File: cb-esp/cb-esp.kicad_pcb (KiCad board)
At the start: 4 copper layers, 25.4 x 55.8 mm, 24 parts, among them P1 CONN_01X07, P2 CONN_01X07, P3 CONN_01X02, SW1 SW_PUSH_SMALL, SW2 SW_PUSH_SMALL, U1 MCP1702, U2 ESP-12E, U3 LY-SK10

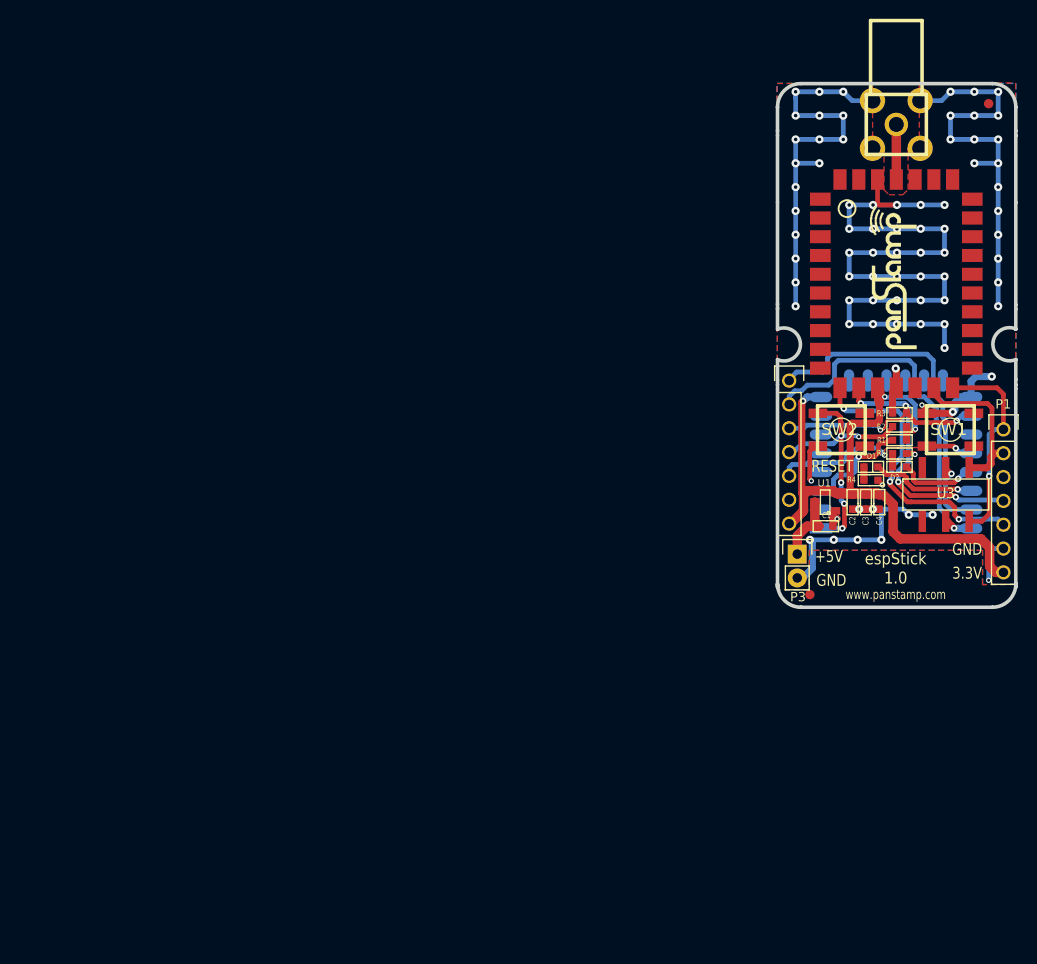
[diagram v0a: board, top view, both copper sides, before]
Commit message: Version 1.0 released
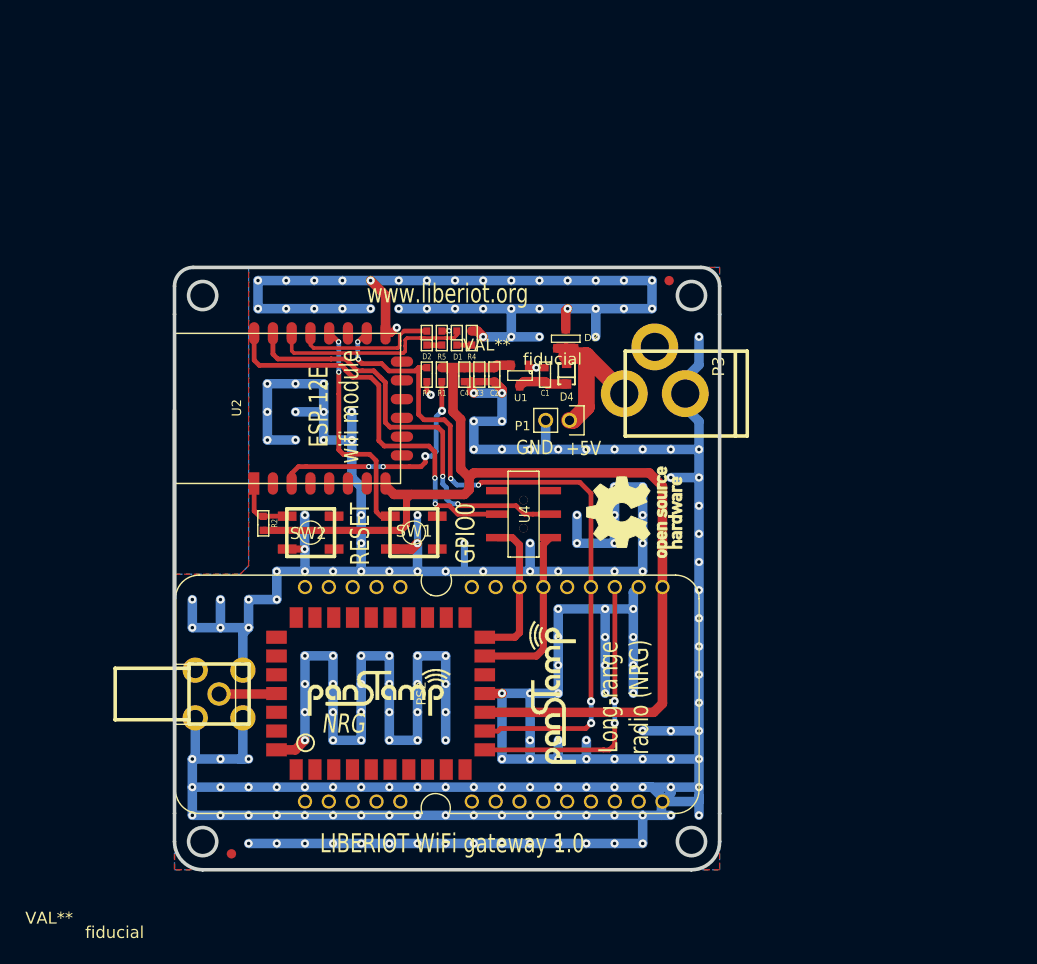
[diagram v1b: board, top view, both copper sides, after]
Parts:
- removed ANT1: ANTENNA, myconnectors:SMA_RightAngle_Tyco
- removed the G*** at (121.9, 83.3)
- removed P2: CONN_01X07, Pin_Headers:Pin_Header_Straight_1x07
- removed the fiducial at (115.8, 109.5)
- removed the fiducial at (134.9, 57.1)
- added D3: D_Schottky_x2_ACom_KKA, mysmd:SOT23, F.Cu at (89.8, 82.2)
- added D4: BAS16, SOD323, F.Cu at (89.9, 85.9)
- added G***: PANSTAMPLOGO, mymods:PANSTAMPLOGO, F.Cu at (62.3, 117.1)
- added G***: PANSTAMPLOGO, mymods:PANSTAMPLOGO, F.Cu at (85.6, 127.5)
- added G***: LOGO, mysmd:oshlogo, F.Cu at (97.1, 100.7)
- added PS2: PANSTAMP_MINIBAT, mymods:minibat, F.Cu at (76.0, 120.1)
- added U4: LY-SK10, LY-SK10, F.Cu at (85.3, 100.9)
- added fiducial: VAL**, mymods:fiducial, F.Cu at (54.2, 137.1)
- added fiducial: VAL**, mymods:fiducial, F.Cu at (100.8, 76.0)
- P1: value CONN_01X07 -> CONN_01X02; footprint Pin_Headers:Pin_Header_Straight_1x07 -> Pin_Headers:Pin_Header_Straight_1x02
- P3: footprint Pin_Headers:Pin_Header_Straight_1x02 -> myconnectors:PWR_3A
- U2: footprint mysmd:ESP-12E -> ESP-12E; moved to F.Cu
- U3: value LY-SK10 -> ANTENNA; footprint mysmd:LY-SK10 -> myconnectors:SMA_RightAngle_Tyco
- moved U3 80.3 mm to (52.9, 120.1), turned to 90 degrees
- moved PS1 70.2 mm to (70.1, 120.0), turned to 90 degrees
- moved R2 68.6 mm to (57.6, 101.9), turned to 270 degrees
- moved U2 60.6 mm to (56.6, 97.6), turned to 90 degrees
- moved SW1 58.2 mm to (73.6, 102.9)
- moved SW2 57.6 mm to (62.6, 102.9)
- moved D2 52.2 mm to (75.0, 82.1), turned to 270 degrees
- moved R3 50.6 mm to (75.0, 86.0), turned to 90 degrees
- moved R5 50.3 mm to (76.6, 82.1), turned to 270 degrees
- moved R1 49.3 mm to (76.6, 86.0), turned to 90 degrees
- moved C4 46.3 mm to (79.0, 86.0)
- moved P1 46.3 mm to (90.2, 90.9), turned to 270 degrees
- moved D1 46.2 mm to (78.2, 82.1), turned to 270 degrees
- moved R4 45.2 mm to (79.8, 82.1), turned to 270 degrees
- moved C3 43.4 mm to (80.6, 86.0)
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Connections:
- P1 pad 1: /PS_RXD -> +5V
- P1 pad 2: /PS_TXD -> GND
- P3 pad 1: Net-(C1-Pad1) -> +5V
- PS1 pad 31: /TOANT -> Net-(PS1-Pad31)
- SW1 pad 1: GND -> /GPIO0
- SW1 pad 2: /GPIO0 -> GND
- U3 pad 1: /PS_TXD -> Net-(PS1-Pad31)
- U3 pad 2: /ESP_RXD -> GND
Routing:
- net GND: track 223.9 -> 720.1 mm, vias 82 -> 216
- net VCC: track 78.9 -> 114.0 mm, vias 3 -> 0
- net /GPIO15: track 51.3 -> 78.2 mm
- net /ESP_RESET: track 29.3 -> 7.83 mm, vias 5 -> 0
- net +5V: track 0.00 -> 19.3 mm
- net Net-(R1-Pad1): track 12.7 -> 25.5 mm, vias 1 -> 4
- net Net-(D1-Pad2): track 13.0 -> 21.7 mm, vias 1 -> 0
- net Net-(D2-Pad2): track 8.47 -> 15.2 mm, vias 1 -> 0
- net Net-(PS1-Pad31): track 0.00 -> 6.14 mm
- net /PS_RXD: track 22.1 -> 16.0 mm, vias 1 -> 0
- net /ESP_RXD: track 39.4 -> 45.3 mm, vias 1 -> 2
- net /TOANT: track 5.87 -> 0.00 mm
- net /ESP_TXD: track 39.4 -> 42.2 mm, vias 1 -> 2
- net Net-(C1-Pad1): track 8.03 -> 5.29 mm
- net /GPIO0: track 22.9 -> 24.6 mm
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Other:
- board size 25.4 x 55.8 mm -> 58.1 x 64.2 mm
- board text added: "ESP-12E wifi module"
- board text added: "GPIO0"
- board text added: "LIBERIOT WiFi gateway 1.0"
- board text added: "Long-range radio (NRG)"
- board text added: "NRG"
- board text added: "www.liberiot.org"
- board text removed: "3.3V"
- board text removed: "espStick 1.0"
- board text removed: "www.panstamp.com"
